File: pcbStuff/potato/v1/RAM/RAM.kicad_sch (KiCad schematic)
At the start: 14 parts, among them U1 74LS138, U10 74LS00, U11 74LS00, U12 74LS74, U13 74LS74, U2 74LS138, U3 74LS04, U4 74LS74, U5 74LS74, U6 74LS74, U7 74LS00, U8 74LS00, U9 74LS00

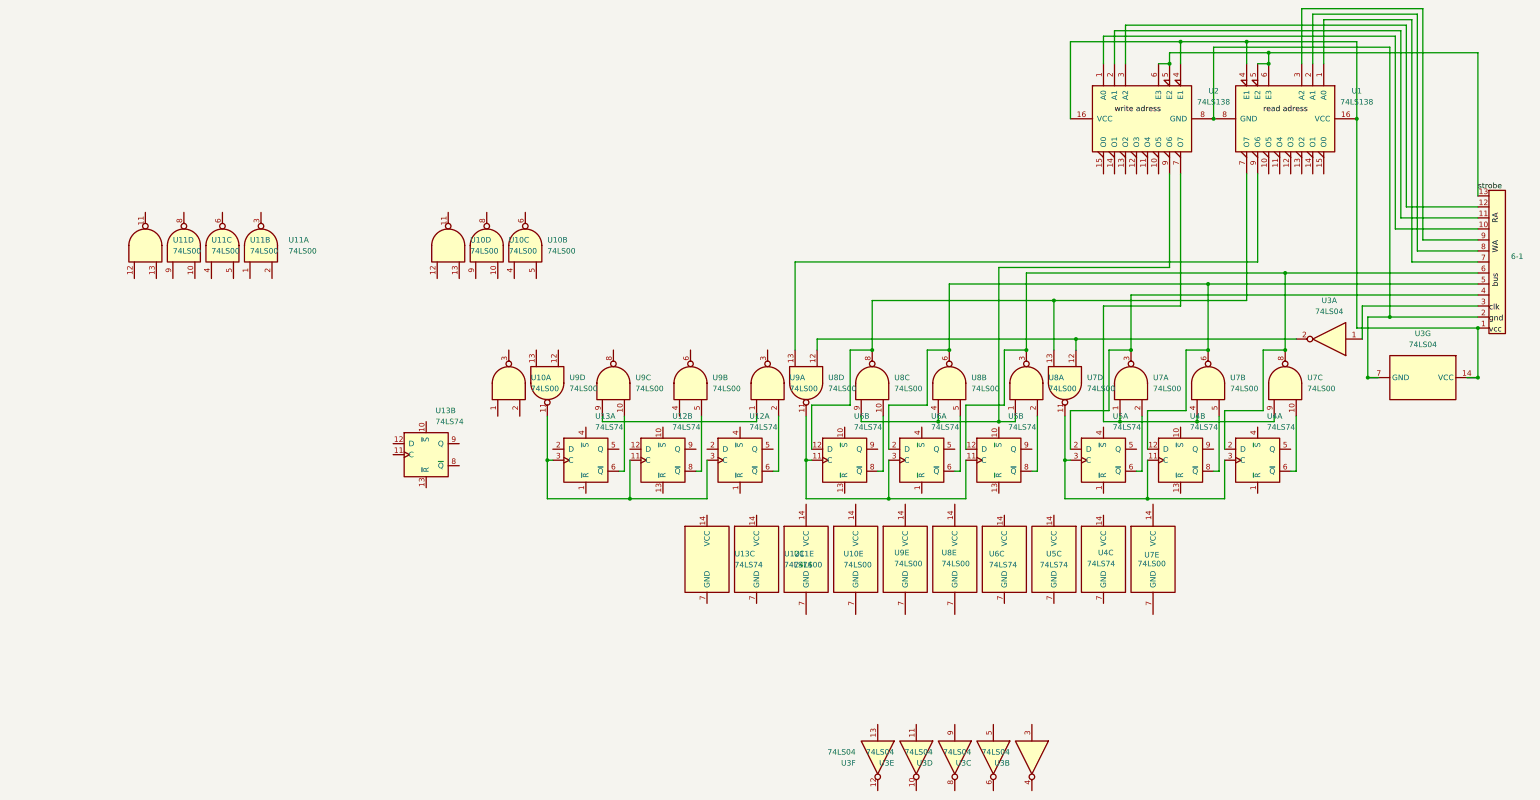
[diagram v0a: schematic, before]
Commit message: holy hell
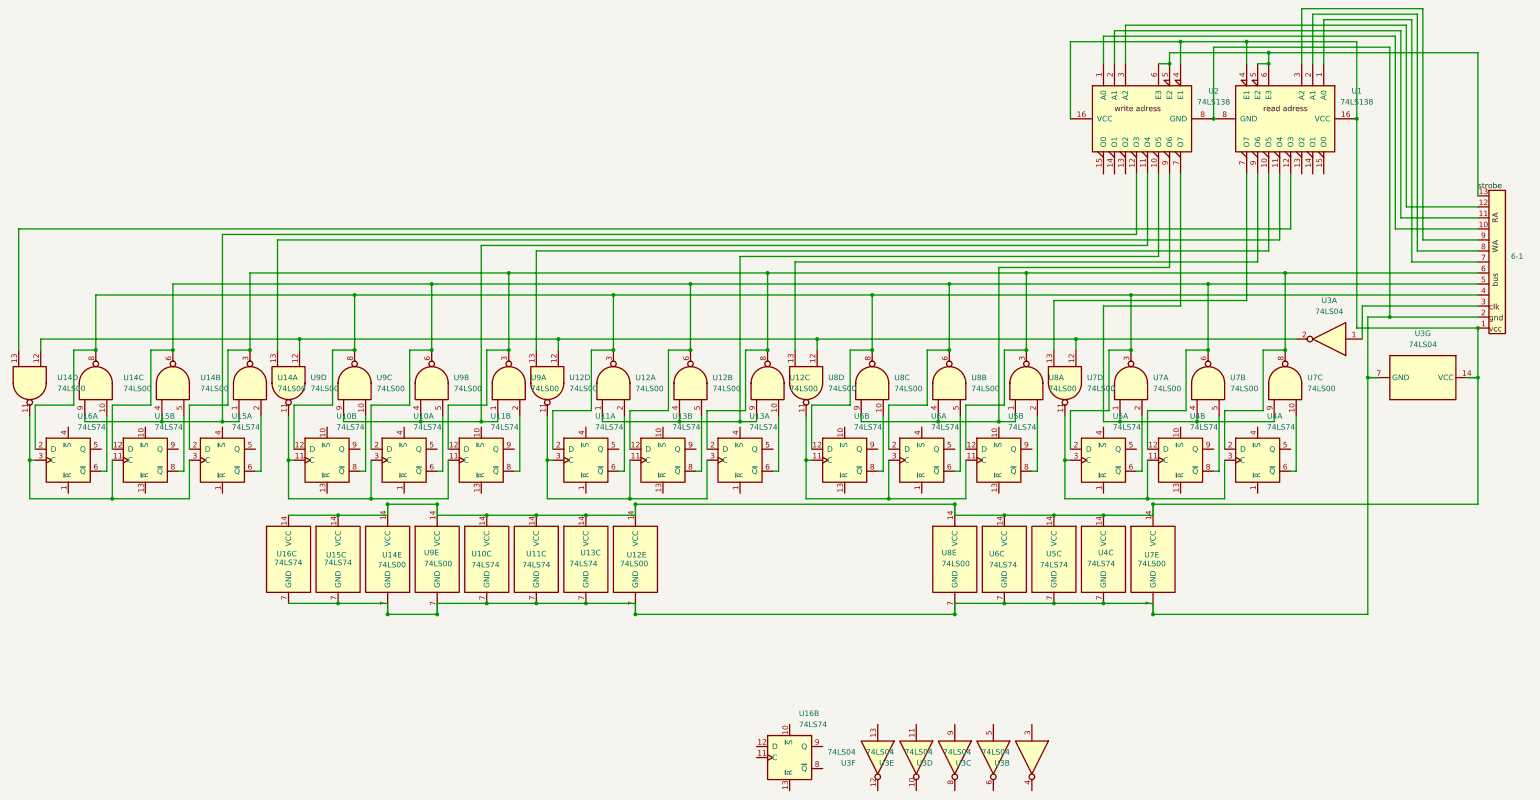
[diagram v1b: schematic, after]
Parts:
- removed U10, U11: 74LS00, symbol 74xx:74LS00
- removed U12: 74LS74, symbol 74xx:74LS74
- added U10, U11, U15, U16: 74LS74, Package_DIP:DIP-14_W7.62mm, symbol 74xx:74LS74
- added U12, U14: 74LS00, Package_DIP:DIP-14_W7.62mm, symbol 74xx:74LS00
- 6-1: footprint (none) -> PotatoComputerV1:6-7Connector
- U1, U2: footprint (none) -> Package_DIP:DIP-16_W7.62mm
- U13, U3, U4, U5, U6, U7, U8, U9: footprint (none) -> Package_DIP:DIP-14_W7.62mm
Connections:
- net at U3.2, U7.12, U8.12: now also U9.12, U12.12, U14.12
- net at U1.7 (O7), U7.13: no longer U6.12 (D), U8.8
- net at U9.1, U9.9: now also U2.11 (O4), U9.4
- net at U9.2: now also U11.8 (~{Q})
- net at U9.3: now also 6-1.6, U13.2 (D), U4.2 (D), U5.12 (D), U7.8, U8.3, U11.12 (D), U12.8, U14.3, U15.2 (D)
- net at 6-1.5, U4.12 (D), U6.2 (D)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: now also U13.12 (D), U9.6, U10.2 (D), U12.6, U14.6, U15.12 (D)
- net at U13.3 (C): now also U13.11 (C), U11.3 (C), U12.11; no longer U9.11
- net at U9.13: now also U1.11 (O4)
- net at 6-1.1, U1.16 (VCC), U1.4 (E1)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: now also U13.14 (VCC), U4.14 (VCC), U5.14 (VCC), U6.14 (VCC), U7.14 (VCC), U8.14 (VCC), U9.14 (VCC), U10.14 (VCC), U11.14 (VCC), U12.14 (VCC), U14.14 (VCC), U15.14 (VCC), U16.14 (VCC)
- net at 6-1.2, U1.8 (GND), U2.8 (GND)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: now also U13.7 (GND), U4.7 (GND), U5.7 (GND), U6.7 (GND), U7.7 (GND), U8.7 (GND), U9.7 (GND), U10.7 (GND), U11.7 (GND), U12.7 (GND), U14.7 (GND), U15.7 (GND), U16.7 (GND)
- net at 6-1.4, U5.2 (D), U7.3: now also U6.12 (D), U8.8, U9.8, U10.12 (D), U11.2 (D), U12.3, U14.8, U16.2 (D)
- net at U1.10 (O5): now also U12.13
- net at U1.12 (O3): now also U14.13
- net at U9.5: now also U10.6 (~{Q})
- net at U13.8 (~{Q}): now also U12.5
- net at U13.6 (~{Q}): now also U12.10; no longer U9.10
- net at U2.10 (O5): now also U12.1, U12.4, U12.9
- net at U2.12 (O3): now also U14.1, U14.4, U14.9
- new net: U11.6 (~{Q}), U12.2
- new net: U10.11 (C), U10.3 (C), U11.11 (C), U9.11
- new net: U10.8 (~{Q}), U9.10
- new net: U14.5, U15.8 (~{Q})
- new net: U14.11, U15.11 (C), U15.3 (C), U16.3 (C)
- new net: U14.10, U16.6 (~{Q})
- new net: U14.2, U15.6 (~{Q})
